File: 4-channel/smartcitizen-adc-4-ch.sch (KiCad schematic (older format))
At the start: 30 parts, among them J1 EXT-V, J2 EXT-V, M1 PINHD-1x10-HEADER, T1 NMOSFET, T2 NMOSFET, U1 ADS1115IDGS

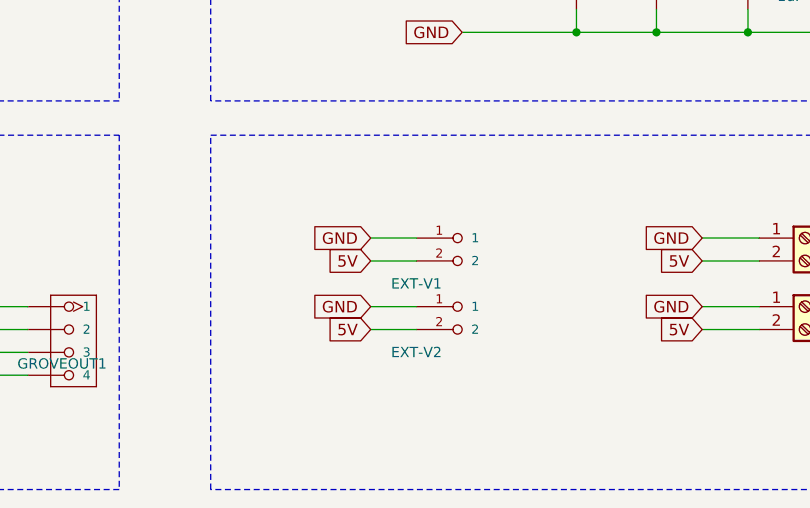
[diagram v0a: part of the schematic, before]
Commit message: 4-channel exports
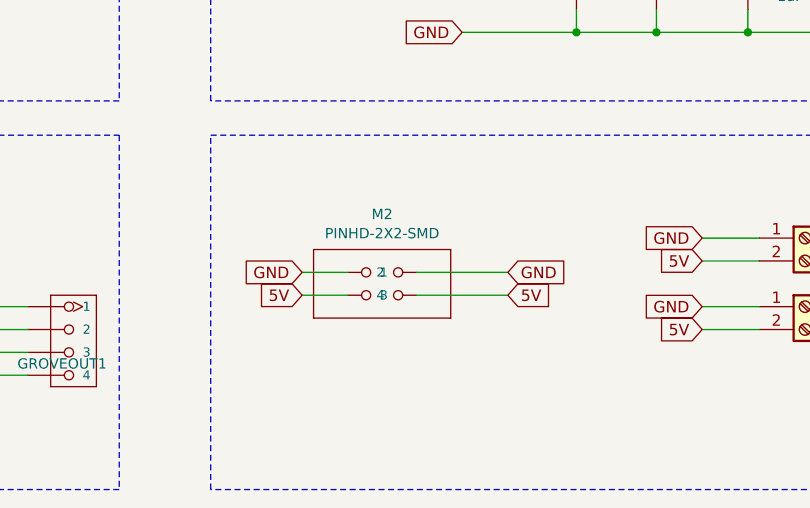
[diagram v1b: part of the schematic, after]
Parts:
- removed EXT-V1, EXT-V2: PINHD-1x02-HEADER, fab:fab-1X02, symbol fab:PINHD-1x02-HEADER
- added M2: PINHD-2X2-SMD, fab-2X02SMD, symbol fab:PINHD-2X2-SMD
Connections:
- net 5V: now also M2.3, M2.4
- net GND: now also M2.1, M2.2
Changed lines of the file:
@@
 Wire Wire Line
 	7550 1950 7900 1950
-Text GLabel 5300 5700 0    50   Input ~ 0
+Text GLabel 5000 5550 0    50   Input ~ 0
 5V
-Text GLabel 5300 5600 0    50   Input ~ 0
-GND
-Text GLabel 5300 5400 0    50   Input ~ 0
+Text GLabel 5000 5450 0    50   Input ~ 0
+GND
+Text GLabel 5900 5550 2    50   Input ~ 0
 5V
-Text GLabel 5300 5300 0    50   Input ~ 0
+Text GLabel 5900 5450 2    50   Input ~ 0
 GND
 Wire Wire Line
@@
 Connection ~ 10250 1900
 $Comp
-L fab:PINHD-1x02-HEADER EXT-V?
-U 1 1 5EFD4E7E
-P 5500 5800
-AR Path="/5F06E2A2/5EFD4E7E" Ref="EXT-V?"  Part="1"
-AR Path="/5F094158/5EFD4E7E" Ref="EXT-V?"  Part="1"
-AR Path="/5EFD4E7E" Ref="EXT-V1"  Part="1"
-F 0 "EXT-V1" H 5500 6100 45  0000 C CNN
-F 1 "PINHD-1x02-HEADER" H 5500 5800 45  0001 C CNN
-F 2 "fab:fab-1X02" H 5530 5950 20  0001 C CNN
-F 3 "" H 5500 5800 50  0001 C CNN
-	1    5500 5800
-	1    0    0    -1
-$EndComp
-$Comp
 L Device:Ferrite_Bead FB?
 U 1 1 5EFD4E78
@@
 $EndComp
 Wire Wire Line
-	5300 5400 5500 5400
-Wire Wire Line
-	5300 5300 5500 5300
-$Comp
-L fab:PINHD-1x02-HEADER EXT-V?
-U 1 1 5EFD4E06
-P 5500 6100
-AR Path="/5F06E2A2/5EFD4E06" Ref="EXT-V?"  Part="1"
-AR Path="/5F094158/5EFD4E06" Ref="EXT-V?"  Part="1"
-AR Path="/5EFD4E06" Ref="EXT-V2"  Part="1"
-F 0 "EXT-V2" H 5500 6400 45  0000 C CNN
-F 1 "PINHD-1x02-HEADER" H 5500 6100 45  0001 C CNN
-F 2 "fab:fab-1X02" H 5530 6250 20  0001 C CNN
-F 3 "" H 5500 6100 50  0001 C CNN
-	1    5500 6100
-	1    0    0    -1
-$EndComp
-Wire Wire Line
-	5300 5700 5500 5700
-Wire Wire Line
-	5300 5600 5500 5600
+	5000 5550 5200 5550
+Wire Wire Line
+	5000 5450 5200 5450
 Wire Wire Line
 	7550 2300 7900 2300
@@
 	1    0    0    -1
 $EndComp
+$Comp
+L fab:PINHD-2X2-SMD M2
+U 1 1 5F086F4A
+P 5400 5550
+F 0 "M2" H 5350 5904 45  0000 C CNN
+F 1 "PINHD-2X2-SMD" H 5350 5820 45  0000 C CNN
+F 2 "fab-2X02SMD" H 5430 5700 20  0001 C CNN
+F 3 "" H 5400 5550 50  0001 C CNN
+	1    5400 5550
+	1    0    0    -1
+$EndComp
+Wire Wire Line
+	5500 5450 5900 5450
+Wire Wire Line
+	5500 5550 5900 5550
 $EndSCHEMATC

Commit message: 4-channel on pcb version
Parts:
- GROVEIN1: value GROVE-CONNECTOR-DIP_4P-2.0_ -> GROVE-CONNECTOR-SMD-90D_4+2P-2.0_; footprint OPL_Connector:HW4-2.0 -> OPL_Connector:HW4-SMD-2.0-90D; symbol OPL_Connector:GROVE-CONNECTOR-DIP_4P-2.0_ -> OPL_Connector:GROVE-CONNECTOR-SMD-90D_4+2P-2.0_; SKU 320110033 -> 320110032
- GROVEOUT1: footprint OPL_Connector:HW4-2.0 -> OPL_Connector:HW4-SMD-2.0-90D; symbol OPL_Connector:GROVE-CONNECTOR-DIP_4P-2.0_ -> OPL_Connector:GROVE-CONNECTOR-SMD-90D_4+2P-2.0_; SKU 320110033 -> 320110032
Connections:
- net GND: now also GROVEIN1.5 (SS1), GROVEIN1.6 (SS2), GROVEOUT1.5 (SS1), GROVEOUT1.6 (SS2)
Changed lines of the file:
@@
 	4600 4700 4600 3150
 $Comp
-L OPL_Connector:GROVE-CONNECTOR-DIP_4P-2.0_ GROVEIN?
+L OPL_Connector:GROVE-CONNECTOR-SMD-90D_4+2P-2.0_ GROVEIN?
 U 1 1 5EFD4D2C
-P 2800 5750
+P 2850 5750
 AR Path="/5F06E2A2/5EFD4D2C" Ref="GROVEIN?"  Part="1"
 AR Path="/5F094158/5EFD4D2C" Ref="GROVEIN?"  Part="1"
 AR Path="/5EFD4D2C" Ref="GROVEIN1"  Part="1"
-F 0 "GROVEIN1" H 2800 5650 45  0000 C CNN
-F 1 "GROVE-CONNECTOR-DIP_4P-2.0_" H 2800 5750 45  0001 C CNN
-F 2 "OPL_Connector:HW4-2.0" H 2830 5900 20  0001 C CNN
-F 3 "" H 2800 5750 50  0001 C CNN
-F 4 "320110033" H 2800 5750 50  0001 C CNN "SKU"
-	1    2800 5750
+F 0 "GROVEIN1" V 3000 5750 45  0000 C CNN
+F 1 "GROVE-CONNECTOR-SMD-90D_4+2P-2.0_" H 2850 5750 45  0001 C CNN
+F 2 "OPL_Connector:HW4-SMD-2.0-90D" H 2880 5900 20  0001 C CNN
+F 3 "" H 2850 5750 50  0001 C CNN
+F 4 "320110032" H 2850 5750 50  0001 C CNN "SKU"
+	1    2850 5750
 	1    0    0    -1
 $EndComp
@@
 GROVE
 $Comp
-L OPL_Connector:GROVE-CONNECTOR-DIP_4P-2.0_ GROVEOUT?
+L OPL_Connector:GROVE-CONNECTOR-SMD-90D_4+2P-2.0_ GROVEOUT?
 U 1 1 5EFD4D38
-P 3950 5750
+P 4000 5750
 AR Path="/5F06E2A2/5EFD4D38" Ref="GROVEOUT?"  Part="1"
 AR Path="/5F094158/5EFD4D38" Ref="GROVEOUT?"  Part="1"
 AR Path="/5EFD4D38" Ref="GROVEOUT1"  Part="1"
-F 0 "GROVEOUT1" H 3950 5650 45  0000 C CNN
-F 1 "GROVE-CONNECTOR-DIP_4P-2.0_" H 3950 5750 45  0001 C CNN
-F 2 "OPL_Connector:HW4-2.0" H 3980 5900 20  0001 C CNN
-F 3 "" H 3950 5750 50  0001 C CNN
-F 4 "320110033" H 3950 5750 50  0001 C CNN "SKU"
-	1    3950 5750
-	1    0    0    -1
-$EndComp
-Wire Wire Line
-	2350 5600 2350 5450
-Wire Wire Line
-	2350 5450 3400 5450
-Wire Wire Line
-	3400 5450 3400 5600
+F 0 "GROVEOUT1" V 4150 5750 45  0000 C CNN
+F 1 "GROVE-CONNECTOR-DIP_4P-2.0_" H 4000 5750 45  0001 C CNN
+F 2 "OPL_Connector:HW4-SMD-2.0-90D" H 4030 5900 20  0001 C CNN
+F 3 "" H 4000 5750 50  0001 C CNN
+F 4 "320110032" H 4000 5750 50  0001 C CNN "SKU"
+	1    4000 5750
+	1    0    0    -1
+$EndComp
 Wire Wire Line
 	3400 5600 3800 5600
@@
 	2350 5600 2650 5600
 Wire Wire Line
-	2450 5700 2450 5550
-Wire Wire Line
-	2450 5550 3300 5550
-Wire Wire Line
-	3300 5550 3300 5700
+	2450 5700 2450 5500
+Wire Wire Line
+	2450 5500 3300 5500
+Wire Wire Line
+	3300 5500 3300 5700
 Wire Wire Line
 	3300 5700 3800 5700
@@
 	2350 5900 2350 6100
 Wire Wire Line
-	2350 6100 3400 6100
+	2350 6100 2850 6100
 Wire Wire Line
 	3400 6100 3400 5900
@@
 GND
 Wire Wire Line
-	1400 5900 2350 5900
+	1400 5900 2050 5900
 Wire Wire Line
 	1400 5800 2450 5800
@@
 Wire Wire Line
 	5500 5550 5900 5550
+Wire Wire Line
+	2850 6050 2850 6100
+Connection ~ 2850 6100
+Wire Wire Line
+	2850 6100 3400 6100
+Wire Wire Line
+	2850 5350 2050 5350
+Wire Wire Line
+	2050 5350 2050 5900
+Connection ~ 2050 5900
+Wire Wire Line
+	2050 5900 2350 5900
+Wire Wire Line
+	2350 5400 3400 5400
+Wire Wire Line
+	2350 5400 2350 5600
+Wire Wire Line
+	3400 5400 3400 5600
+Wire Wire Line
+	2850 5350 2850 5450
+Wire Wire Line
+	4000 5450 4000 5350
+Wire Wire Line
+	4000 5350 2850 5350
+Connection ~ 2850 5350
+Wire Wire Line
+	3400 6100 4000 6100
+Wire Wire Line
+	4000 6100 4000 6050
+Connection ~ 3400 6100
 $EndSCHEMATC

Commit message: Move traces out of screw, move components to bottom layer for SMD
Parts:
- C1: LCSC (none) -> C1944
- C2: LCSC (none) -> C24497
- C3, C4: LCSC (none) -> C1848
- FB1, FB2: LCSC (none) -> C21517
- R1, R2, R3, R4, R5, R6: LCSC (none) -> C17902
- T1: LCSC (none) -> C431497
- T2: LCSC (none) -> NCE2304
- U1: LCSC (none) -> C37593
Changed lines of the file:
@@
 F 2 "fab-SOT-23" H 2530 1700 20  0001 C CNN
 F 3 "https://www.mouser.es/datasheet/2/308/NDS355AN-D-1813055.pdf" H 2500 1550 50  0001 C CNN
+F 4 "C431497" V 2500 1550 50  0001 C CNN "LCSC"
 	1    2500 1550
 	0    1    1    0
@@
 F 2 "fab-R1206FAB" H 2230 1500 20  0001 C CNN
 F 3 "" H 2200 1350 50  0001 C CNN
+F 4 "C17902" V 2200 1350 50  0001 C CNN "LCSC"
 	1    2200 1350
 	0    1    1    0
@@
 F 2 "fab-R1206FAB" H 2780 1500 20  0001 C CNN
 F 3 "" H 2750 1350 50  0001 C CNN
+F 4 "C17902" V 2750 1350 50  0001 C CNN "LCSC"
 	1    2750 1350
 	0    1    1    0
@@
 F 2 "fab-SOT-23" H 2530 2500 20  0001 C CNN
 F 3 "https://www.mouser.es/datasheet/2/308/NDS355AN-D-1813055.pdf" H 2500 2350 50  0001 C CNN
+F 4 "NCE2304" V 2500 2350 50  0001 C CNN "LCSC"
 	1    2500 2350
 	0    1    1    0
@@
 F 2 "fab-R1206FAB" H 2780 2300 20  0001 C CNN
 F 3 "" H 2750 2150 50  0001 C CNN
+F 4 "C17902" V 2750 2150 50  0001 C CNN "LCSC"
 	1    2750 2150
 	0    1    1    0
@@
 F 2 "fab-R1206FAB" H 2230 2300 20  0001 C CNN
 F 3 "" H 2200 2150 50  0001 C CNN
+F 4 "C17902" V 2200 2150 50  0001 C CNN "LCSC"
 	1    2200 2150
 	0    1    1    0
@@
 F 2 "fab:fab-C1206FAB" H 9030 1750 20  0001 C CNN
 F 3 "https://product.tdk.com/info/en/catalog/datasheets/mlcc_commercial_general_en.pdf?ref_disty=digikey" H 9000 1600 50  0001 C CNN
+F 4 "C1848" V 9000 1600 50  0001 C CNN "LCSC"
 	1    9000 1600
 	0    1    1    0
@@
 F 2 "fab-R1206FAB" H 10280 1800 20  0001 C CNN
 F 3 "" H 10250 1650 50  0001 C CNN
+F 4 "C17902" V 10250 1650 50  0001 C CNN "LCSC"
 	1    10250 1650
 	0    1    1    0
@@
 F 2 "fab:fab-R1206FAB" V 7380 4400 50  0001 C CNN
 F 3 "https://product.tdk.com/info/en/catalog/datasheets/beads_commercial_signal_mmz2012_en.pdf" H 7450 4400 50  0001 C CNN
+F 4 "C21517" V 7450 4400 50  0001 C CNN "LCSC"
 	1    7450 4400
 	0    1    1    0
@@
 F 2 "fab:fab-C1206FAB" H 6950 4200 50  0001 C CNN
 F 3 "https://product.tdk.com/info/en/catalog/datasheets/mlcc_commercial_general_en.pdf?ref_disty=digikey" H 6950 4200 50  0001 C CNN
+F 4 "C1848" V 6950 4200 50  0001 C CNN "LCSC"
 	1    6950 4200
 	0    1    1    0
@@
 F 2 "fab:fab-R1206FAB" V 7380 3900 50  0001 C CNN
 F 3 "https://product.tdk.com/info/en/catalog/datasheets/beads_commercial_signal_mmz2012_en.pdf" H 7450 3900 50  0001 C CNN
+F 4 "C21517" V 7450 3900 50  0001 C CNN "LCSC"
 	1    7450 3900
 	0    1    1    0
@@
 F 2 "fab-R1206FAB" H 10180 2700 20  0001 C CNN
 F 3 "" H 10150 2550 50  0001 C CNN
+F 4 "C17902" V 10150 2550 50  0001 C CNN "LCSC"
 	1    10150 2550
 	0    1    1    0
@@
 F 2 "Package_SO:TSSOP-10_3x3mm_P0.5mm" H 9600 1600 50  0001 C CNN
 F 3 "http://www.ti.com/lit/ds/symlink/ads1113.pdf" H 9550 1200 50  0001 C CNN
+F 4 "C37593" H 9600 2100 50  0001 C CNN "LCSC"
 	1    9600 2100
 	1    0    0    -1
@@
 F 2 "fab:fab-C1206FAB" H 6580 4350 20  0001 C CNN
 F 3 "https://api.kemet.com/component-edge/download/datasheet/C1206C104KARACTU.pdf" H 6550 4200 50  0001 C CNN
+F 4 "C24497" V 6550 4200 50  0001 C CNN "LCSC"
 	1    6550 4200
 	0    1    1    0
@@
 F 2 "fab:fab-C1206FAB" H 6230 4350 20  0001 C CNN
 F 3 "https://www.mouser.es/datasheet/2/447/UPY-GPHC_X7R_6.3V-to-50V_18-1154002.pdf" H 6200 4200 50  0001 C CNN
+F 4 "C1944" V 6200 4200 50  0001 C CNN "LCSC"
 	1    6200 4200
 	0    1    1    0
